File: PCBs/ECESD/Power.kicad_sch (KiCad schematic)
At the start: 22 parts, among them U100 TLV62569DBV, U101 TLV62569DBV

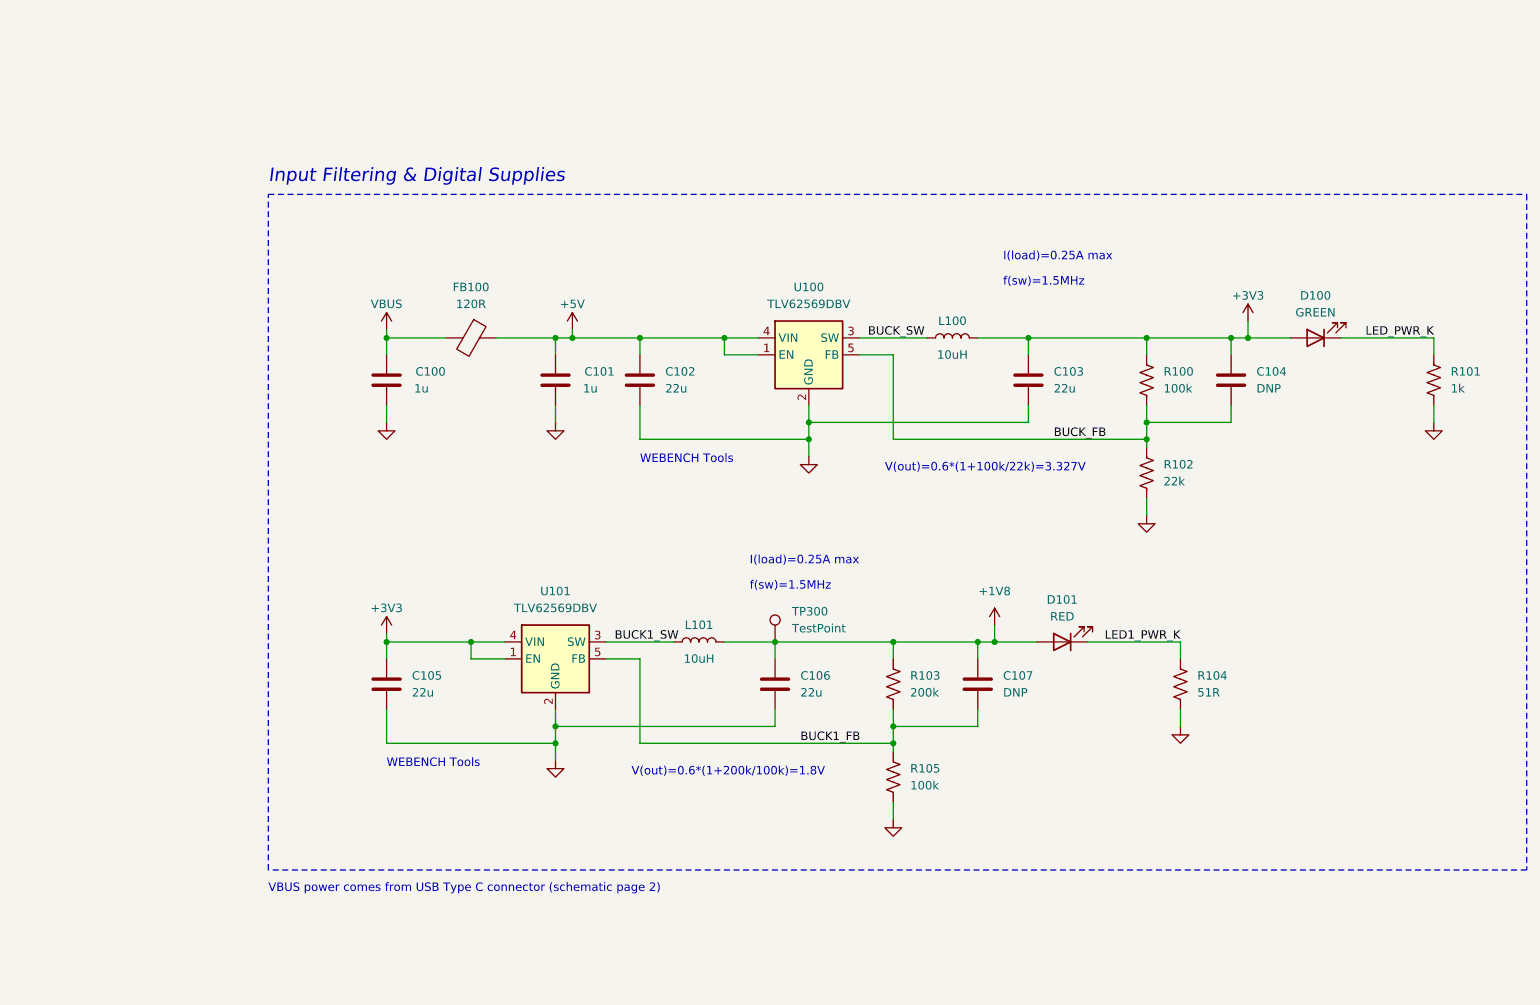
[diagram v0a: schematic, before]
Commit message: Changed PCB 1
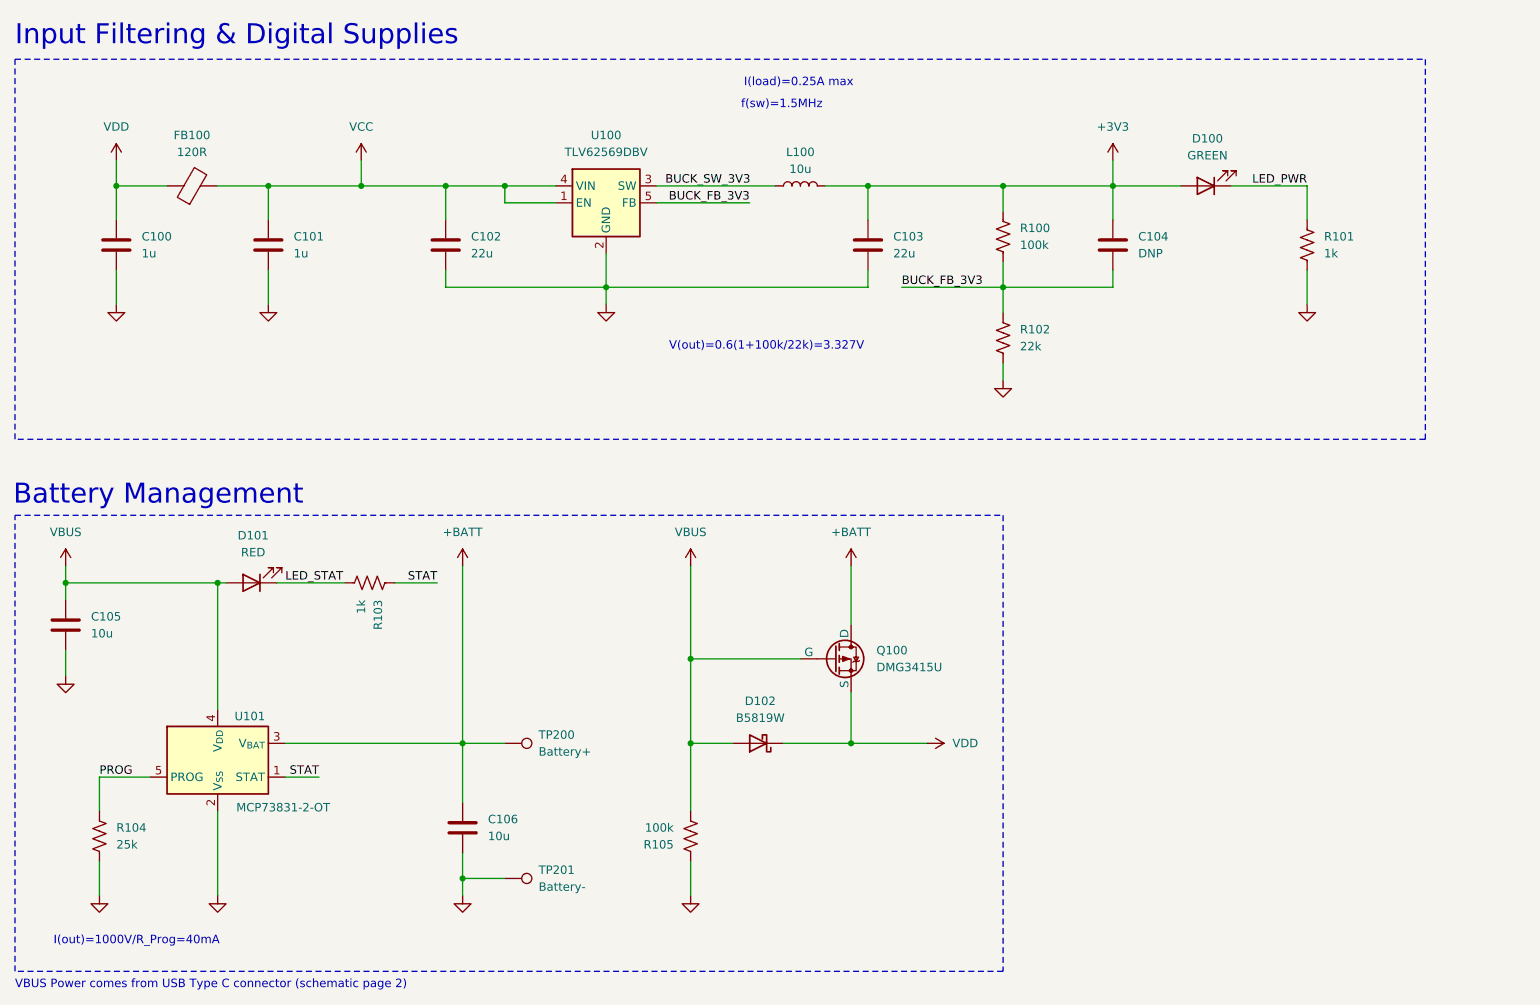
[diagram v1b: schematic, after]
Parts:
- removed C107: DNP, Capacitor_SMD:C_0603_1608Metric_Pad1.08x0.95mm_HandSolder, symbol Device:C
- removed FB100: 120R, Inductor_SMD:L_0603_1608Metric_Pad1.05x0.95mm_HandSolder, symbol Nemesis-MixSigPCB-rescue:Ferrite_Bead-Device
- removed L101: 10uH, VLS4015CX_100M_H:IND_VLS4015CX-100M-H, symbol Device:L
- removed TP300: TestPoint, TestPoint:TestPoint_Pad_D1.0mm, symbol Connector:TestPoint
- removed U101: TLV62569DBV, Package_TO_SOT_SMD:SOT-23-5, symbol Regulator_Switching:TLV62569DBV
- added D102: B5819W, Diode_SMD:D_SOD-123, symbol Device:D_Schottky
- added FB100: 120R, Inductor_SMD:L_0603_1608Metric_Pad1.05x0.95mm_HandSolder, symbol Device:FerriteBead
- added Q100: DMG3415U, Package_TO_SOT_SMD:SOT-23, symbol Simulation_SPICE:PMOS
- added TP200: Battery+, TestPoint:TestPoint_Pad_3.0x3.0mm, symbol Connector:TestPoint
- added TP201: Battery-, TestPoint:TestPoint_Pad_3.0x3.0mm, symbol Connector:TestPoint
- added U101: MCP73831-2-OT, Package_TO_SOT_SMD:SOT-23-5, symbol Battery_Management:MCP73831-2-OT
- C105, C106: value 22u -> 10u; footprint Capacitor_SMD:C_0805_2012Metric_Pad1.18x1.45mm_HandSolder -> Capacitor_SMD:C_0603_1608Metric_Pad1.08x0.95mm_HandSolder
- L100: value 10uH -> 10u; footprint VLS4015CX_100M_H:IND_VLS4015CX-100M-H -> Power Inductor:IND_VLS4015CX-100M-H
- R103: value 200k -> 1k
- R104: value 51R -> 25k
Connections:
- net +3V3: no longer C105.1
- net GND: now also R105.1, TP201.1, U101.2 (V_{SS}); no longer R105.2
- net VBUS: now also C105.1, D101.2 (A), R105.2, D102.2 (A), Q100.2 (G), U101.4 (V_{DD}); no longer C100.1
- removed net +1V8: C106.1, D101.2 (A), R103.1
- net +5V renamed VCC
- net VCC: now also FB100.2
- net BUCK1_FB renamed LED_STAT
- net LED_STAT: now also D101.1 (K); no longer R105.1
- net BUCK_FB renamed BUCK_FB_3V3
- net BUCK_SW renamed BUCK_SW_3V3
- net LED1_PWR_K renamed PROG
- net PROG: now also U101.5 (PROG); no longer D101.1 (K)
- net LED_PWR_K renamed LED_PWR
- new net +BATT: C106.1, Q100.1 (D), TP200.1, U101.3 (V_{BAT})
- new net STAT: R103.1, U101.1 (STAT)
- new net VDD: C100.1, D102.1 (K), FB100.1, Q100.3 (S)
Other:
- note added: "Battery Management"
- note added: "I(out)=1000V/R_Prog=40mA"
- note added: "V(out)=0.6(1+100k/22k)=3.327V"
- note added: "VBUS Power comes from USB Type C connector (schematic page 2)"
- note removed: "V(out)=0.6*(1+100k/22k)=3.327V"
- note removed: "V(out)=0.6*(1+200k/100k)=1.8V"
- note removed: "VBUS power comes from USB Type C connector (schematic page 2)"
- note removed: "WEBENCH Tools"
